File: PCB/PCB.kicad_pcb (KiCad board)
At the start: 2 copper layers, 100 x 115.5 mm, 14 parts

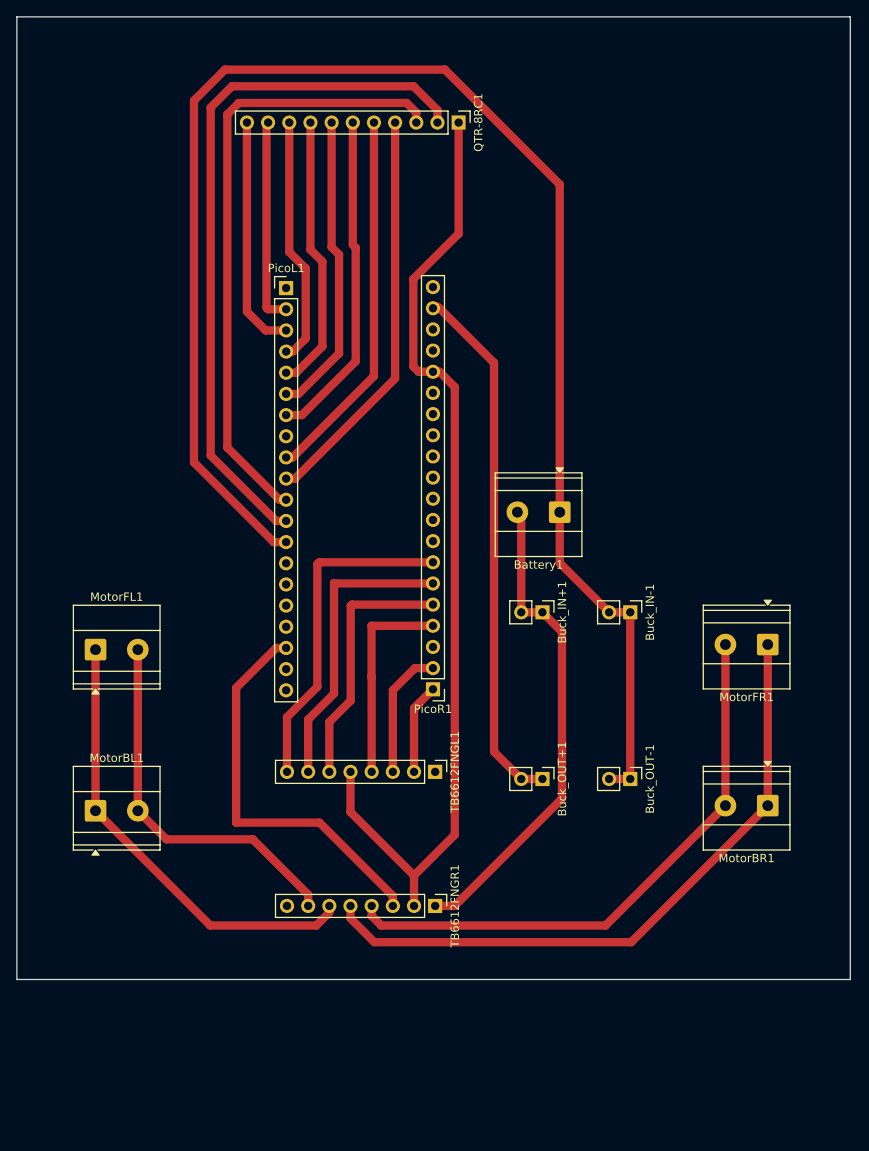
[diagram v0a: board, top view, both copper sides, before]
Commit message: centralized
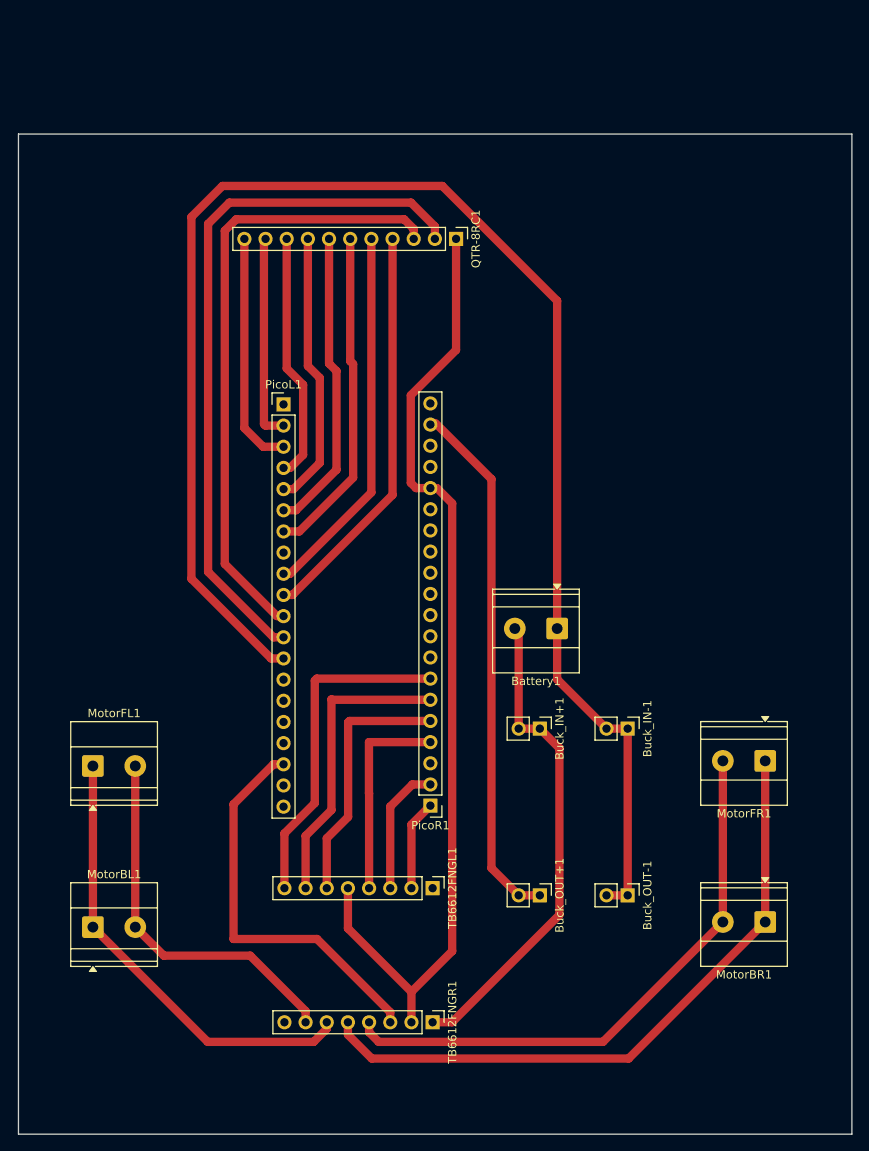
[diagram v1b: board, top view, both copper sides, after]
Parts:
- moved TB6612FNGL1 14.0 mm to (49.9, 104.5)
- moved Battery1 14.0 mm to (64.8, 73.4)
- moved PicoL1 14.0 mm to (32.0, 46.5)
- moved QTR-8RC1 14.0 mm to (52.7, 26.6)
- moved Buck_IN+1 14.0 mm to (62.7, 85.4)
- moved Buck_IN-1 14.0 mm to (73.3, 85.4)
- moved Buck_OUT+1 14.0 mm to (62.7, 105.4)
- moved Buck_OUT-1 14.0 mm to (73.3, 105.4)
- moved MotorBL1 14.0 mm to (9.13, 109.2)
- moved MotorBR1 14.0 mm to (89.8, 108.6)
- moved MotorFL1 14.0 mm to (9.13, 89.9)
- moved MotorFR1 14.0 mm to (89.8, 89.3)
- moved PicoR1 14.0 mm to (49.6, 94.6)
- moved TB6612FNGR1 14.0 mm to (49.9, 120.6)
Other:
- board size 100 x 115.5 mm -> 100 x 120 mm

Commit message: auto
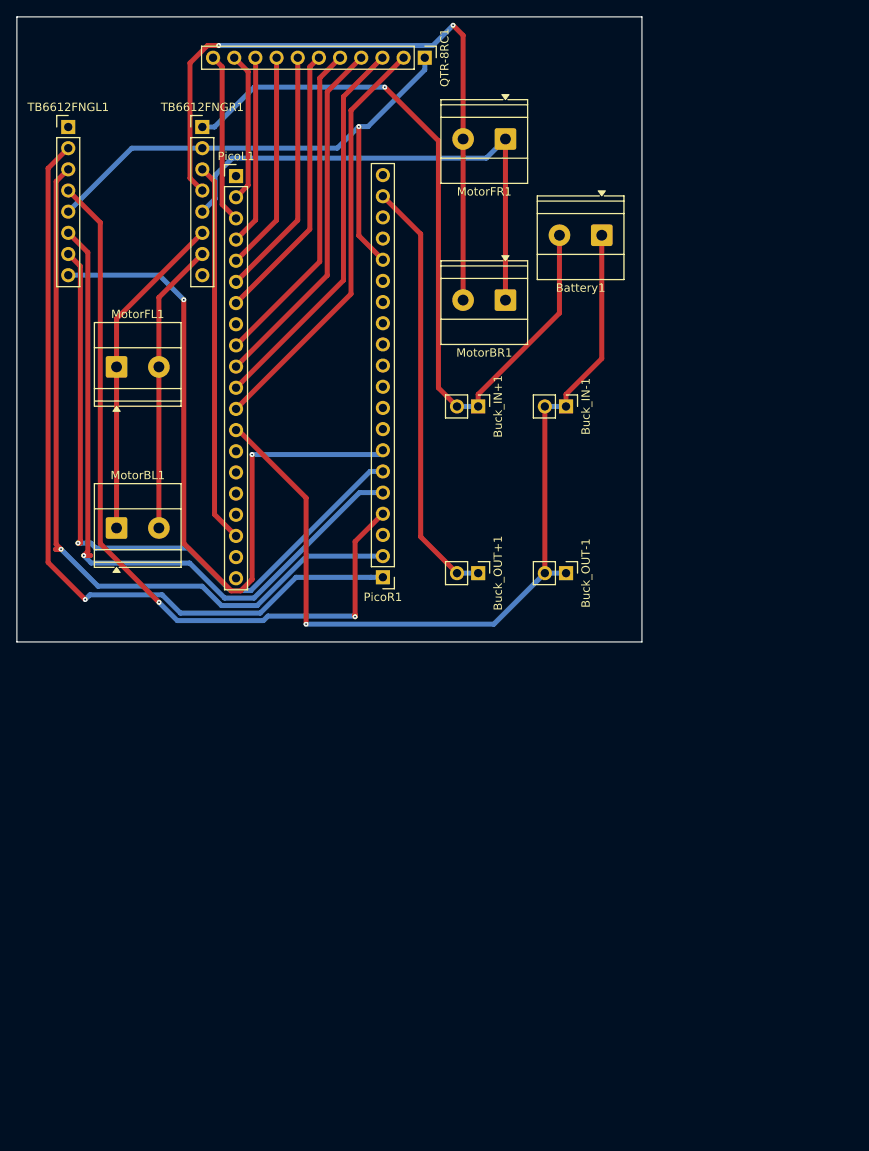
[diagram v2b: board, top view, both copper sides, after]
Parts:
- moved TB6612FNGR1 110.9 mm to (22.3, 13.2), turned to 0 degrees
- moved TB6612FNGL1 101.3 mm to (6.16, 13.2), turned to 0 degrees
- moved MotorFR1 80.9 mm to (58.6, 14.7)
- moved MotorBR1 80.9 mm to (58.6, 34.0)
- moved MotorBL1 48.0 mm to (12.0, 61.3)
- moved MotorFL1 48.0 mm to (12.0, 42.0)
- moved Battery1 47.5 mm to (70.2, 26.2)
- moved Buck_IN+1 39.4 mm to (55.3, 46.7)
- moved Buck_IN-1 39.4 mm to (65.9, 46.7)
- moved Buck_OUT+1 39.4 mm to (55.3, 66.7)
- moved Buck_OUT-1 39.4 mm to (65.9, 66.7)
- moved PicoR1 28.0 mm to (43.9, 67.2)
- moved PicoL1 28.0 mm to (26.3, 19.1)
- moved QTR-8RC1 22.1 mm to (48.9, 4.90)
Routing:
- net Net-(PicoR1-Pin_1): track 10.8 -> 95.6 mm, vias 0 -> 1
- net GND: track 188.4 -> 105.5 mm, vias 0 -> 1
- net Net-(PicoR1-Pin_2): track 15.7 -> 92.8 mm, vias 0 -> 1
- net Net-(PicoR1-Pin_4): track 24.9 -> 93.2 mm, vias 0 -> 2
- net Net-(PicoR1-Pin_5): track 30.9 -> 84.7 mm, vias 0 -> 1
- net /3V3_OUT: track 117.4 -> 68.4 mm, vias 0 -> 1
- net Net-(PicoR1-Pin_7): track 40.4 -> 86.3 mm, vias 0 -> 2
- net Net-(PicoR1-Pin_6): track 35.8 -> 81.4 mm, vias 0 -> 1
- net Net-(PicoL1-Pin_12): track 85.0 -> 50.5 mm
- net VCC: track 58.6 -> 92.9 mm, vias 0 -> 1
- net Net-(PicoL1-Pin_11): track 74.5 -> 46.9 mm
- net Net-(MotorBR1-Pin_1): track 78.9 -> 61.0 mm
- net Net-(MotorBL1-Pin_1): track 54.5 -> 39.7 mm
- net Net-(MotorBR1-Pin_2): track 69.4 -> 82.8 mm, vias 0 -> 2
- net /BuckOut: track 63.4 -> 51.4 mm
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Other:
- board size 100 x 120 mm -> 75 x 75 mm

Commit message: 100x100
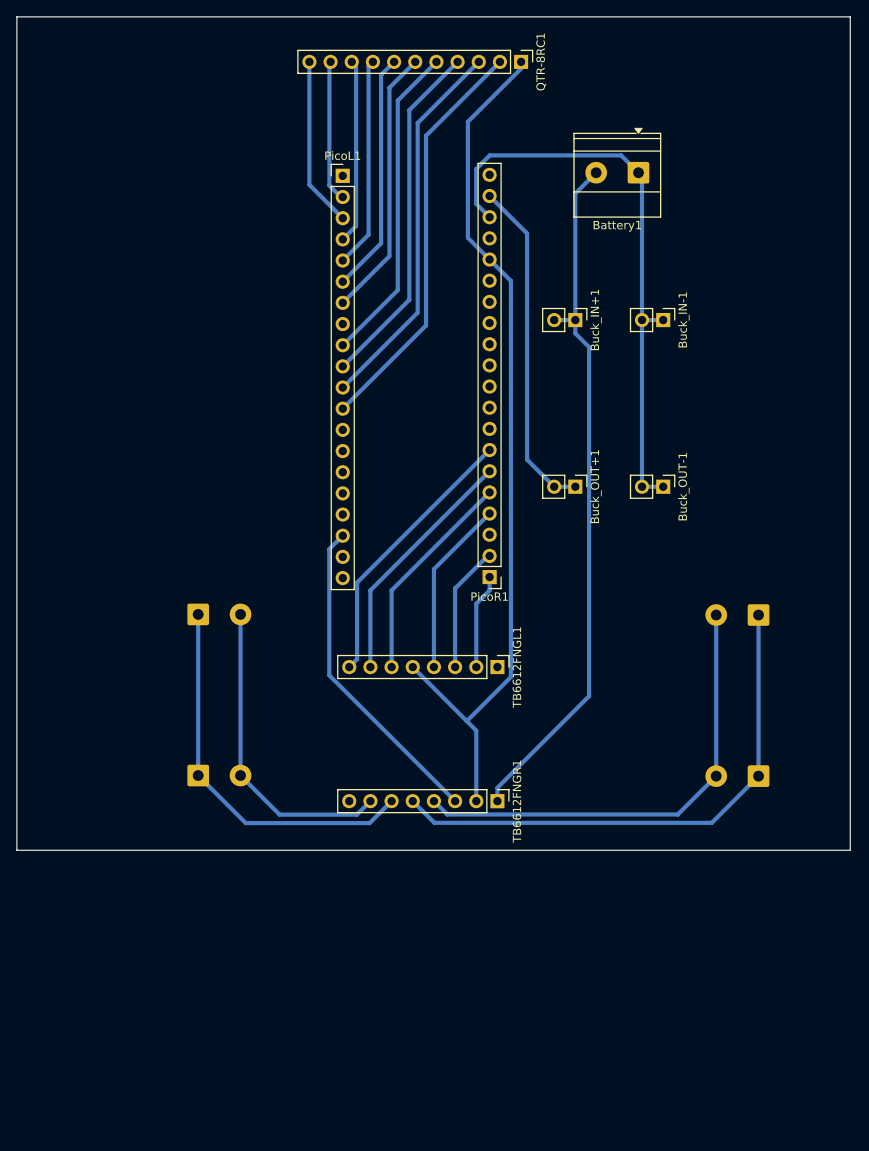
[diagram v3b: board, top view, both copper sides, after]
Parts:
- MotorBL1, MotorBR1, MotorFL1, MotorFR1: moved to B.Cu
- moved TB6612FNGR1 88.3 mm to (57.7, 94.1), turned to -90 degrees
- moved TB6612FNGL1 82.8 mm to (57.7, 78.0), turned to -90 degrees
- moved MotorFR1 82.3 mm to (89.0, 91.1)
- moved MotorFL1 50.0 mm to (21.8, 91.0)
- moved MotorBR1 48.5 mm to (89.0, 71.8)
- moved Buck_IN+1 15.6 mm to (67.0, 36.4)
- moved Buck_OUT+1 15.6 mm to (67.0, 56.4)
- moved Buck_IN-1 15.6 mm to (77.5, 36.4)
- moved Buck_OUT-1 15.6 mm to (77.5, 56.4)
- moved MotorBL1 14.3 mm to (21.8, 71.7)
- moved PicoL1 12.8 mm to (39.1, 19.1)
- moved PicoR1 12.8 mm to (56.7, 67.2)
- moved QTR-8RC1 11.6 mm to (60.5, 5.40)
- moved Battery1 8.70 mm to (74.6, 18.7)
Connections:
- PicoL1 pad 13: GND -> unconnected-(PicoL1-Pin_13-Pad13)
- PicoR1 pad 18: unconnected-(PicoR1-Pin_18-Pad18) -> GND
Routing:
- net Net-(PicoR1-Pin_1): track 95.6 -> 11.5 mm, vias 1 -> 0
- net Net-(PicoR1-Pin_2): track 92.8 -> 15.2 mm, vias 1 -> 0
- net Net-(PicoR1-Pin_4): track 93.2 -> 21.2 mm, vias 2 -> 0
- net Net-(PicoR1-Pin_5): track 84.7 -> 25.8 mm, vias 1 -> 0
- net Net-(PicoR1-Pin_7): track 86.3 -> 33.0 mm, vias 2 -> 0
- net Net-(PicoR1-Pin_6): track 81.4 -> 29.4 mm, vias 1 -> 0
- net /3V3_OUT: track 68.4 -> 105.3 mm, vias 1 -> 0
- net GND: track 105.5 -> 70.4 mm, vias 1 -> 0
- net Net-(MotorBR1-Pin_2): track 82.8 -> 55.8 mm, vias 2 -> 0
- net /BuckOut: track 51.4 -> 40.6 mm
- net VCC: track 92.9 -> 84.2 mm, vias 1 -> 0
- net GND18: track 45.7 -> 38.8 mm
- net Net-(MotorBL1-Pin_1): track 39.7 -> 46.0 mm
- net Net-(MotorBR1-Pin_1): track 61.0 -> 64.2 mm
- net Net-(MotorBL1-Pin_2): track 35.0 -> 37.5 mm
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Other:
- board size 75 x 75 mm -> 100 x 100 mm
- board text added: "MADE BY : HUZAIFA BAGHOOR"
